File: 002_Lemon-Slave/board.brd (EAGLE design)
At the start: 85.1 x 67 mm, 60 parts, among them IC1 74HC595N, IC2 74HC595N, IC3 74HC595N, IC4 7805TV, Q1 14,7456, U1 ATTINY85-20P, X1 MKDSN1,5/2-5,08, X2 MKDSN1,5/2-5,08, X3 MKDSN1,5/2-5,08

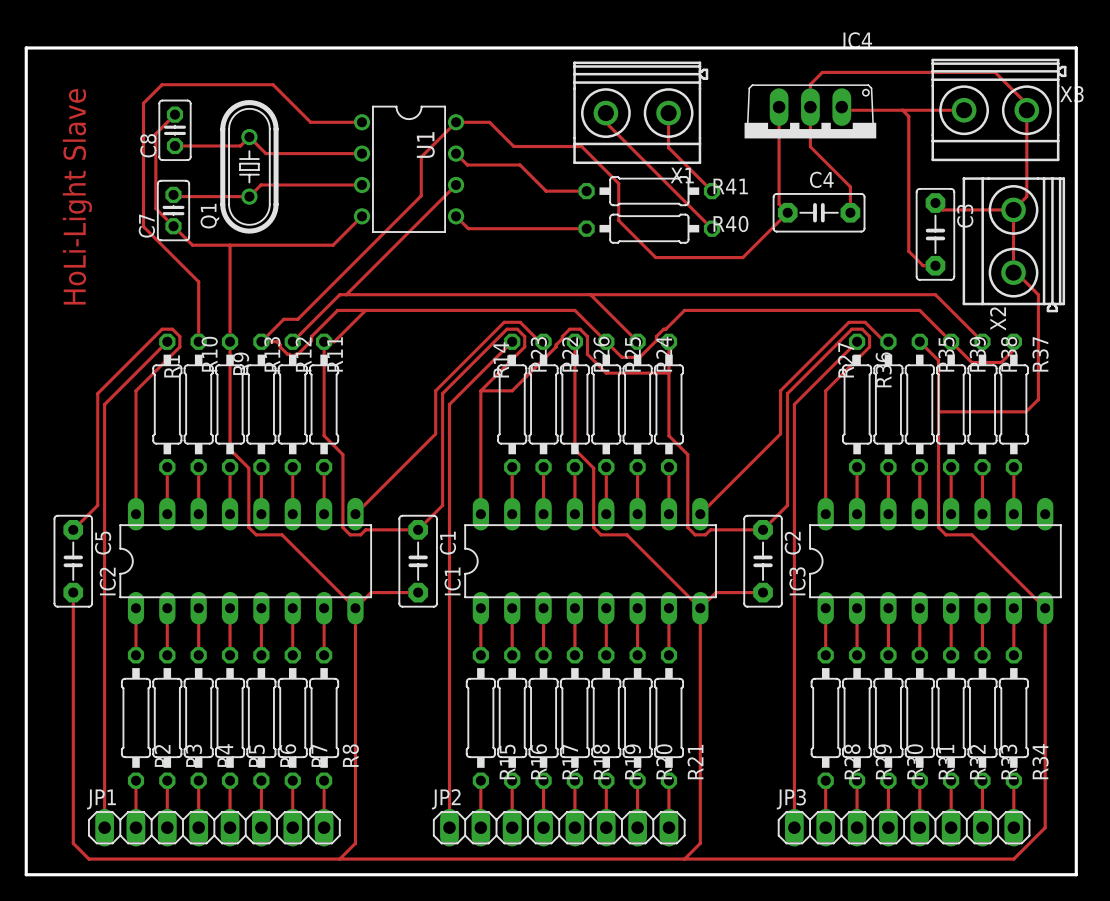
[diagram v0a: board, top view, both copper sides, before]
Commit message: update lemon light main controller
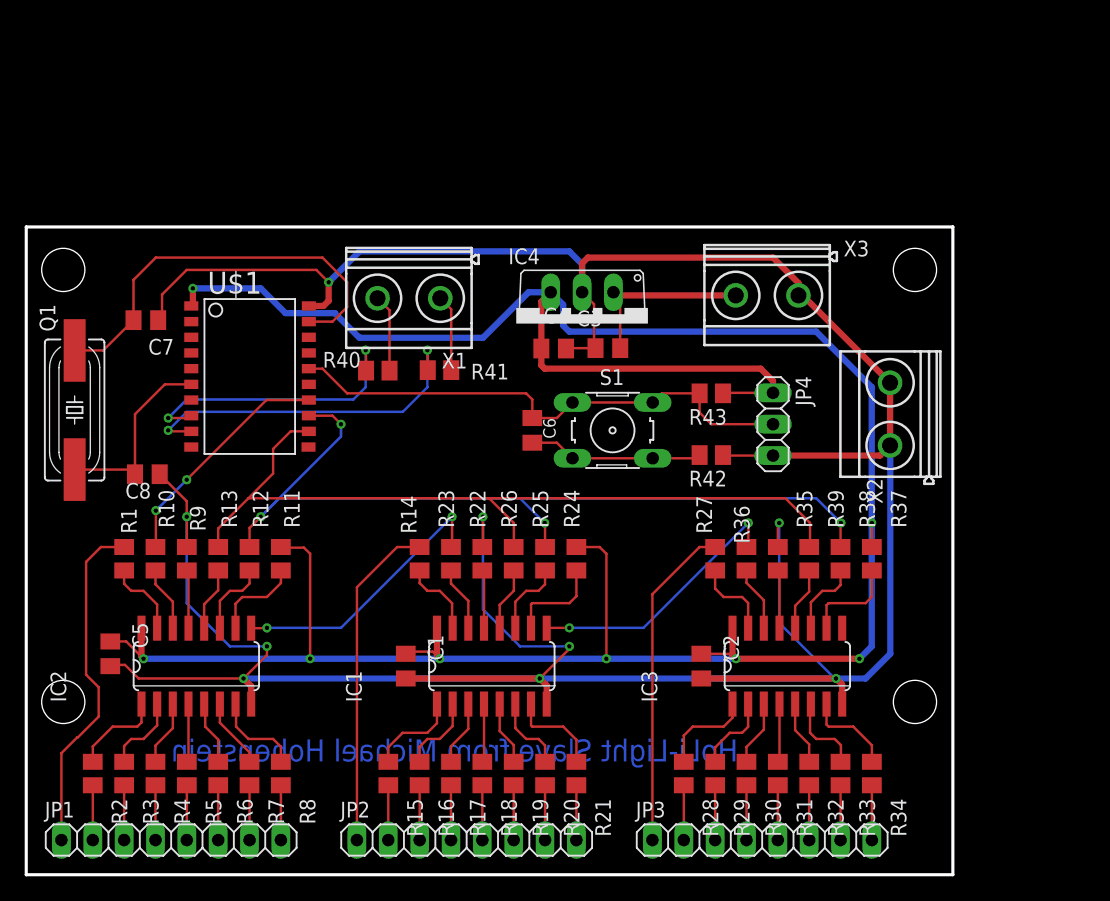
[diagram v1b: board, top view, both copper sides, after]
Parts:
- removed U1: ATTINY85-20P, attiny25_45_85:PDIP08_300MIL
- added C6: 4,7nF, rcl:C0805K
- added JP4: (no value), pinhead:1X03
- added R42: 1K, resistor:M0805
- added R43: 10K, resistor:M0805
- added S1: (no value), switch-omron:B3F-10XX
- added U$1: ATTINY406, My_AVRs:SO20L
- C1, C2, C3, C4, C5: device capacitor-wima:C5B3 -> rcl:C0805K
- C7, C8: value 22pF -> 12pF; device resistor:C025-025X050 -> rcl:C0805K
- IC1, IC2, IC3: value 74HC595N -> 74HC595D; device 74xx-eu:DIL16 -> 74xx-eu:SO16
- Q1: device crystal:HC49/S -> crystal:SM49
- R1, R10, R11, R12, R13, R14, R15, R16, R17, R18, R19, R2, R20, R21, R22, R23, R24, R25, R26, R27, R28, R29, R3, R30, R31, R32, R33, R34, R35, R36, R37, R38, R39, R4, R5, R6, R7, R8, R9: device resistor:0207/10 -> resistor:M0805
- R40, R41: value 500 -> 100; device resistor:0207/10 -> resistor:M0805
- X1, X2, X3: value MKDSN1,5/2-5,08 -> (none)
- moved C3 28.1 mm to (47.1, 42.7), turned to 0 degrees
- moved C8 27.9 mm to (9.81, 32.5), turned to 0 degrees
- moved R40 24.8 mm to (28.5, 40.8)
- moved Q1 24.3 mm to (3.92, 37.6), turned to 270 degrees
- moved C4 24.2 mm to (42.7, 42.6)
- moved IC4 23.8 mm to (45.0, 44.6)
- moved X3 23.8 mm to (60.0, 47.0)
- moved X1 23.8 mm to (31.0, 46.7)
- moved R41 22.3 mm to (33.5, 40.9)
- moved X2 17.2 mm to (70.0, 37.3)
- moved R39 17.0 mm to (63.4, 25.6)
- moved R27 17.0 mm to (55.8, 25.6)
- moved R35 17.0 mm to (60.9, 25.6)
- moved R37 17.0 mm to (68.5, 25.6)
- moved R38 17.0 mm to (66.0, 25.6)
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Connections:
- new net N$68: R13.1, R26.1, R39.1, U$1.12
- new net N$75: C6.1, JP4.2, R43.2, S1.1, S1.2, U$1.16
- new net N$76: C6.2, R42.2, S1.3, S1.4
- net +5V: now also JP4.1, R43.1, U$1.1; no longer R13.1, R26.1, R39.1, U1.8
- net GND: now also JP4.3, R42.1, U$1.20; no longer U1.4
- net N$67: now also U$1.13; no longer U1.6
- net N$69: now also U$1.8; no longer U1.5
- net N$70: now also U$1.9; no longer U1.7
- net N$73: now also U$1.14; no longer U1.1
- net N$74: now also U$1.19; no longer U1.3
- net N$78: now also U$1.6; no longer U1.2
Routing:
- net +5V: track 318.3 -> 216.0 mm, vias 0 -> 8
- net GND: track 358.5 -> 276.6 mm, vias 0 -> 9
- net N$68: track 0.00 -> 66.4 mm
- net N$75: track 0.00 -> 42.9 mm
- net N$73: track 40.8 -> 19.1 mm, vias 0 -> 2
- net N$74: track 15.7 -> 33.5 mm
- net N$70: track 11.8 -> 29.0 mm, vias 0 -> 2
- net N$56: track 41.5 -> 26.6 mm
- net N$35: track 41.5 -> 26.9 mm
- net N$76: track 0.00 -> 14.2 mm
- net N$14: track 41.5 -> 27.8 mm
- net N$69: track 11.0 -> 23.7 mm, vias 0 -> 2
- net N$72: track 24.3 -> 14.8 mm
- net N$66: track 12.9 -> 6.27 mm
- net N$67: track 77.0 -> 71.1 mm, vias 0 -> 4
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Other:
- board size 85.1 x 67 mm -> 75.1 x 52.5 mm
- board text added: "GND"
- board text added: "HoLi-Light Slave from Michael Hohenstein"
- board text added: "Rx"
- board text added: "Tx"
- board text added: "VCC"
- board text removed: "HoLi-Light Slave"
